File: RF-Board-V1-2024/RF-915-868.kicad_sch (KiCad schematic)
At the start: 10 parts, among them J4 UART, J5 Conn_Coaxial, U5 MAX-M10S

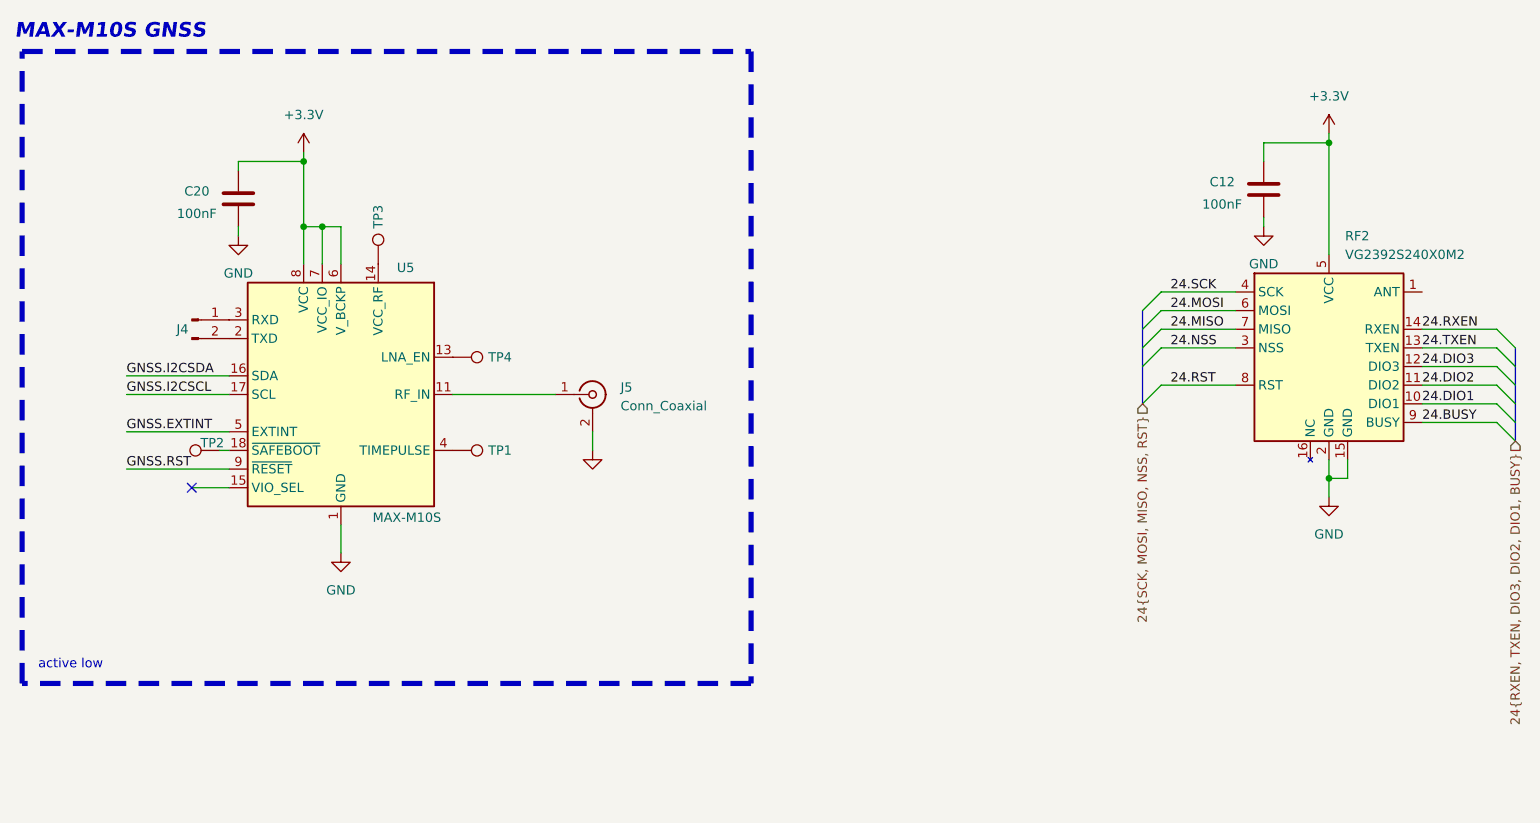
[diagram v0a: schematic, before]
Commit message: i think schematic is done for now
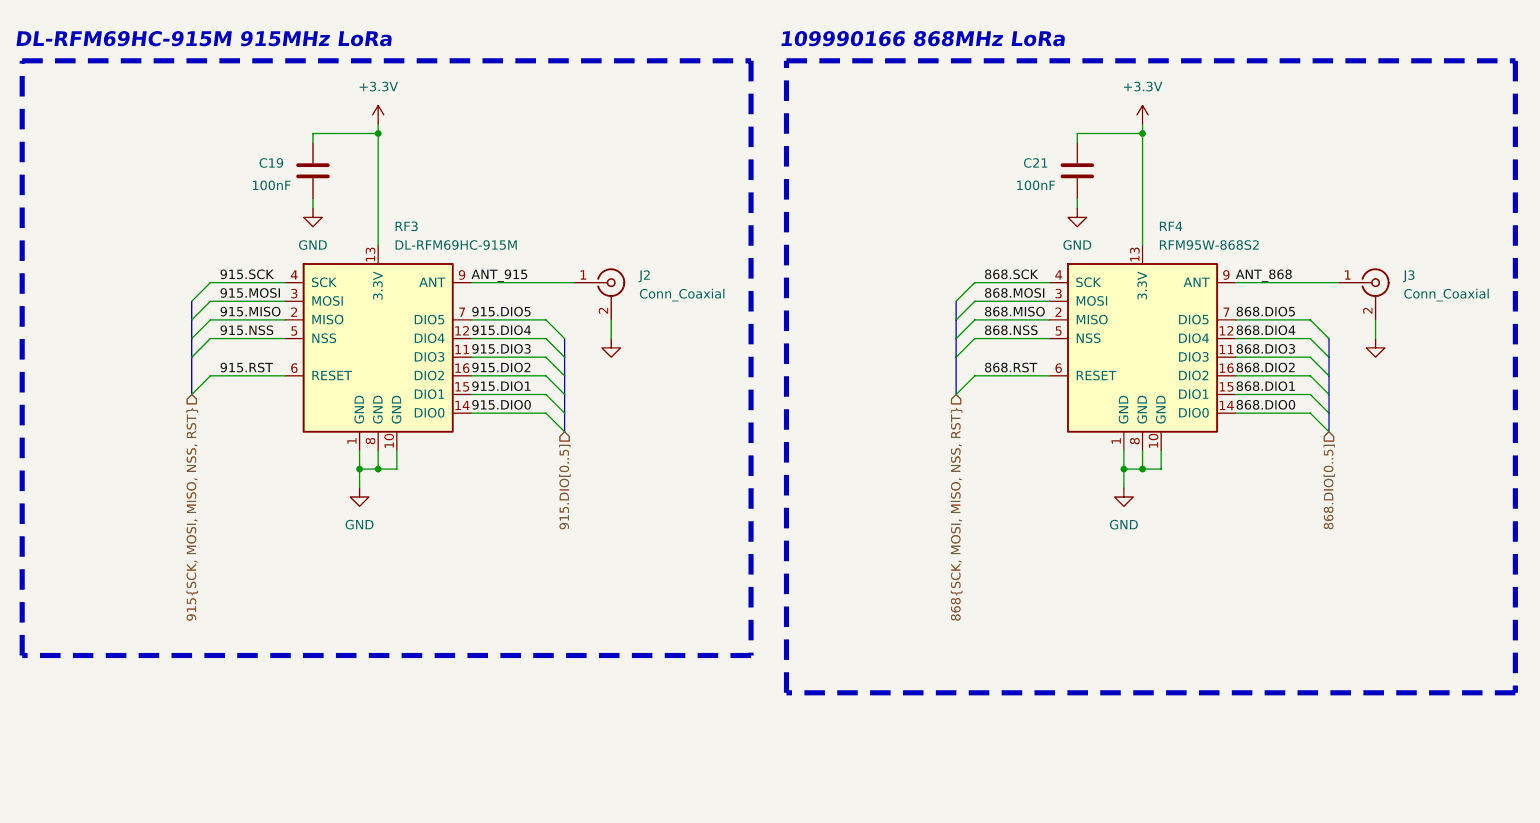
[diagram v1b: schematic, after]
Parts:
- removed C12, C20: 100nF, symbol Device:C
- removed J4: UART, symbol Connector:Conn_01x02_Pin
- removed J5: Conn_Coaxial, footprints:TAOGLAS_EMPCB.SMAFSTJ.B.HT, symbol Connector:Conn_Coaxial
- removed RF2: VG2392S240X0M2, symbol ecocad_lib_symbols:Vollgo_2.4GHz
- removed TP1, TP2, TP3, TP4: TestPoint, symbol Connector:TestPoint
- removed U5: MAX-M10S, RF_GPS:ublox_MAX, symbol RF_GPS:MAX-M10S
- added C19, C21: 100nF, symbol Device:C
- added J2, J3: Conn_Coaxial, footprints:TAOGLAS_EMPCB.SMAFSTJ.B.HT, symbol Connector:Conn_Coaxial
- added RF3: DL-RFM69HC-915M, RF_Module:HOPERF_RFM9XW_THT, symbol RF_Module:RFM69HCW
- added RF4: RFM95W-868S2, symbol RF_Module:RFM95W-868S2
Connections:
- net +3.3V: now also C19.2, C21.2, RF3.13 (3.3V), RF4.13 (3.3V)
- net GND: now also C19.1, C21.1, J2.2 (Ext), J3.2 (Ext), RF3.1 (GND), RF3.10 (GND), RF3.8 (GND), RF4.1 (GND), RF4.10 (GND), RF4.8 (GND)
- new net 868.DIO0: RF4.14 (DIO0)
- new net 868.DIO1: RF4.15 (DIO1)
- new net 868.DIO2: RF4.16 (DIO2)
- new net 868.DIO3: RF4.11 (DIO3)
- new net 868.DIO4: RF4.12 (DIO4)
- new net 868.DIO5: RF4.7 (DIO5)
- new net 868.MISO: RF4.2 (MISO)
- new net 868.MOSI: RF4.3 (MOSI)
- new net 868.NSS: RF4.5 (NSS)
- new net 868.RST: RF4.6 (RESET)
- new net 868.SCK: RF4.4 (SCK)
- new net 915.DIO0: RF3.14 (DIO0)
- new net 915.DIO1: RF3.15 (DIO1)
- new net 915.DIO2: RF3.16 (DIO2)
- new net 915.DIO3: RF3.11 (DIO3)
- new net 915.DIO4: RF3.12 (DIO4)
- new net 915.DIO5: RF3.7 (DIO5)
- new net 915.MISO: RF3.2 (MISO)
- new net 915.MOSI: RF3.3 (MOSI)
- new net 915.NSS: RF3.5 (NSS)
- new net 915.RST: RF3.6 (RESET)
- new net 915.SCK: RF3.4 (SCK)
- new net ANT_868: J3.1 (In), RF4.9 (ANT)
- new net ANT_915: J2.1 (In), RF3.9 (ANT)
- no-connect marks 1 -> 0
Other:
- note added: "109990166 868MHz LoRa"
- note added: "DL-RFM69HC-915M 915MHz LoRa"
- note removed: "MAX-M10S GNSS"
- note removed: "active low"
- title: (none) -> RF 868MHz 915MHz
